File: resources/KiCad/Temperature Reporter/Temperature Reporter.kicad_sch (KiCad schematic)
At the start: 11 parts, among them U1 ESP32-C3-0.42-OLED, U2 DS18B20, U3 DS18B20

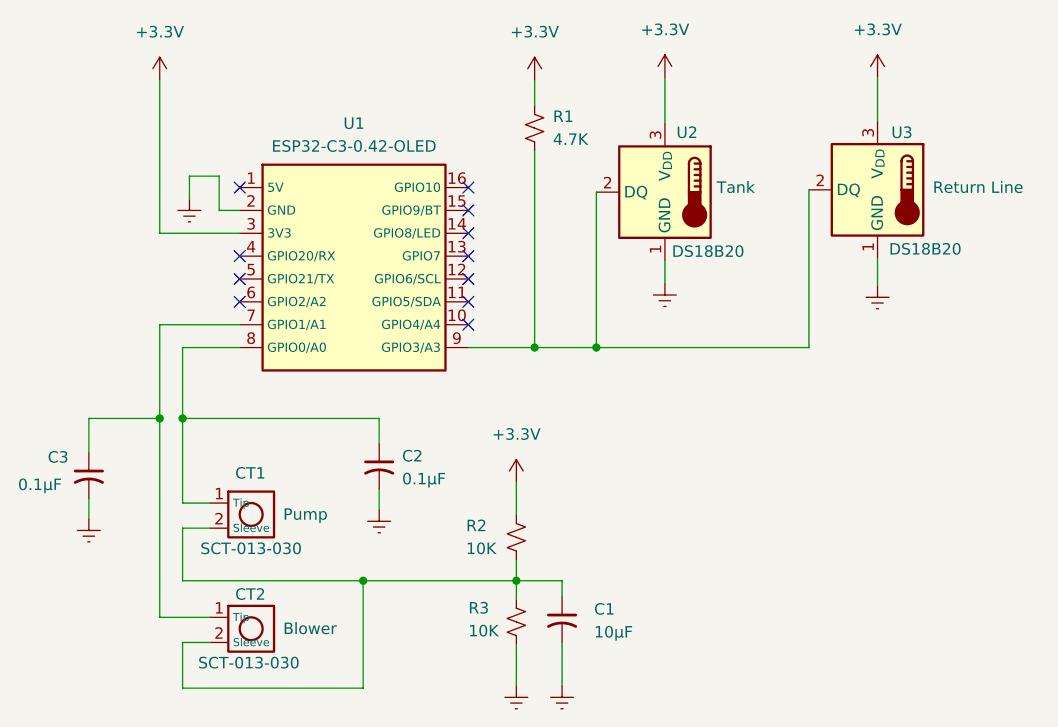
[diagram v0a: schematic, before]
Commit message: updated schematic
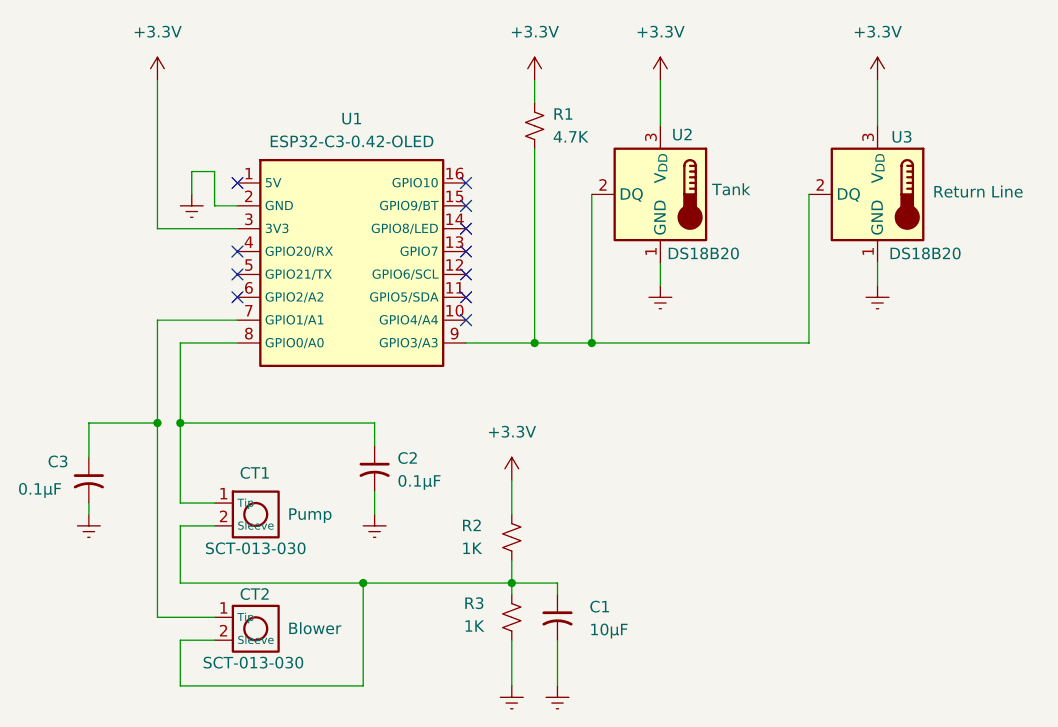
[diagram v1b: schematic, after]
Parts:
- R2, R3: value 10K -> 1K
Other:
- moved on the sheet: C1, C2, C3, CT1, CT2, R2, R3, U1, U2, U3
